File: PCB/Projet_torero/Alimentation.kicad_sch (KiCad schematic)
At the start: 17 parts, among them IC501 MP1475SGJ-P, J2 Conn_01x02, SW3 SW_DPDT_x2, U2 BU33SD5WG-TR

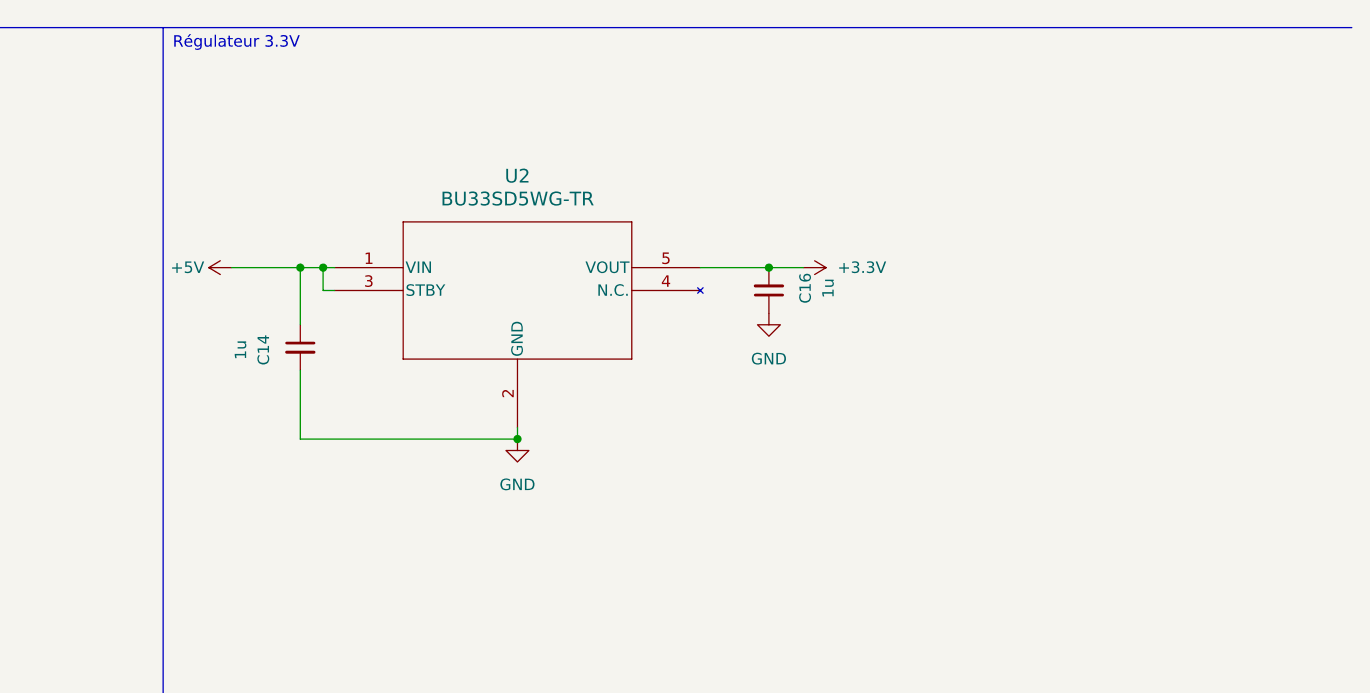
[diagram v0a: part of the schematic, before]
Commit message: review sch
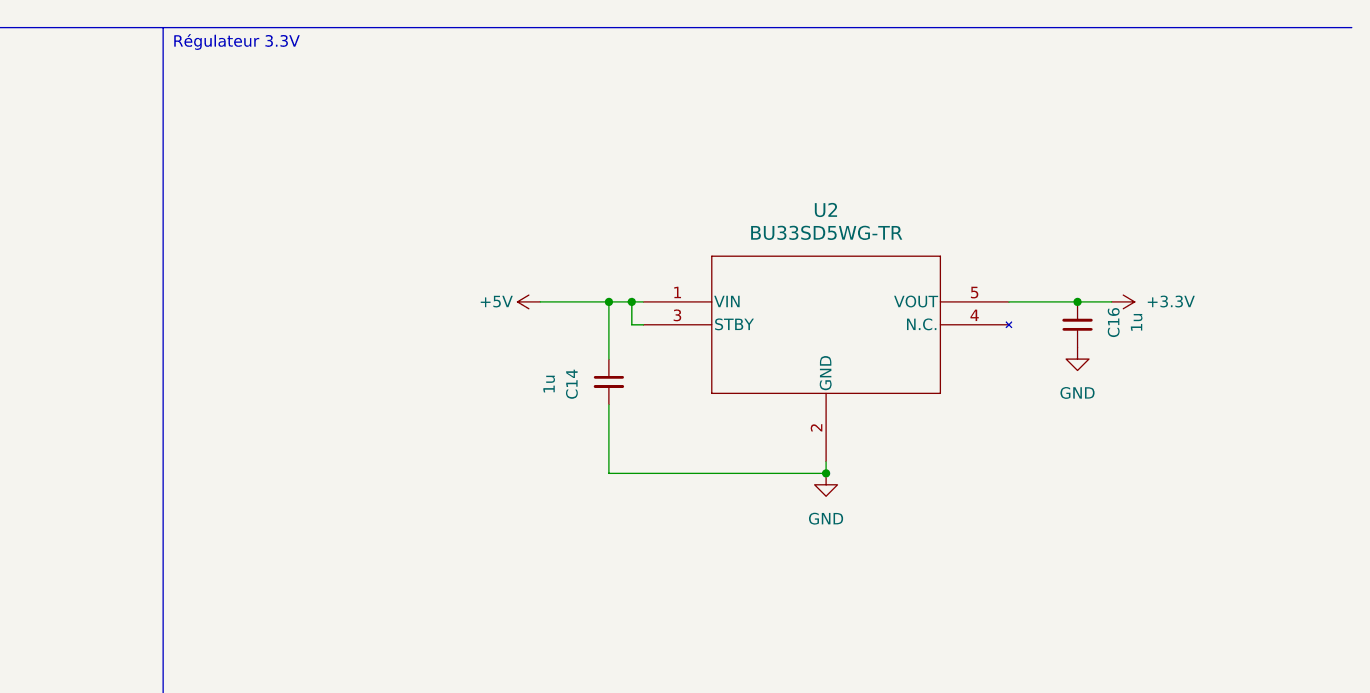
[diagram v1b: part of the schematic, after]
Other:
- moved on the sheet: C14, C16, U2
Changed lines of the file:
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@@
 	(paper "A4")
 	(junction
-		(at 171.45 116.84)
+		(at 205.74 120.65)
 		(diameter 0)
 		(color 0 0 0 0)
@@
 	)
 	(junction
-		(at 168.91 116.84)
+		(at 203.2 120.65)
 		(diameter 0)
 		(color 0 0 0 0)
 	)
 	(junction
-		(at 220.98 116.84)
+		(at 255.27 120.65)
 		(diameter 0)
 		(color 0 0 0 0)
@@
 	)
 	(junction
-		(at 193.04 135.89)
+		(at 227.33 139.7)
 		(diameter 0)
 		(color 0 0 0 0)
@@
 	(wire
 		(pts
-			(xy 168.91 116.84) (xy 168.91 123.19)
+			(xy 203.2 120.65) (xy 203.2 127)
 		)
 		(stroke
@@
 	(wire
 		(pts
-			(xy 168.91 135.89) (xy 193.04 135.89)
+			(xy 203.2 139.7) (xy 227.33 139.7)
 		)
 		(stroke
@@
 	(wire
 		(pts
-			(xy 168.91 128.27) (xy 168.91 135.89)
+			(xy 203.2 132.08) (xy 203.2 139.7)
 		)
 		(stroke
@@
 	(wire
 		(pts
-			(xy 220.98 116.84) (xy 224.79 116.84)
+			(xy 255.27 120.65) (xy 259.08 120.65)
 		)
 		(stroke
@@
 	(wire
 		(pts
-			(xy 213.36 116.84) (xy 220.98 116.84)
+			(xy 247.65 120.65) (xy 255.27 120.65)
 		)
 		(stroke
@@
 	(wire
 		(pts
-			(xy 168.91 116.84) (xy 171.45 116.84)
+			(xy 203.2 120.65) (xy 205.74 120.65)
 		)
 		(stroke
@@
 	(wire
 		(pts
-			(xy 193.04 134.62) (xy 193.04 135.89)
+			(xy 227.33 138.43) (xy 227.33 139.7)
 		)
 		(stroke
@@
 	(wire
 		(pts
-			(xy 171.45 116.84) (xy 171.45 119.38)
+			(xy 205.74 120.65) (xy 205.74 123.19)
 		)
 		(stroke
@@
 	(wire
 		(pts
-			(xy 161.29 116.84) (xy 168.91 116.84)
+			(xy 195.58 120.65) (xy 203.2 120.65)
 		)
 		(stroke
@@
 	(wire
 		(pts
-			(xy 171.45 119.38) (xy 172.72 119.38)
+			(xy 205.74 123.19) (xy 207.01 123.19)
 		)
 		(stroke
@@
 	(wire
 		(pts
-			(xy 171.45 116.84) (xy 172.72 116.84)
+			(xy 205.74 120.65) (xy 207.01 120.65)
 		)
 		(stroke
@@
 	(symbol
 		(lib_id "power:+3.3V")
-		(at 224.79 116.84 270)
+		(at 259.08 120.65 270)
 		(unit 1)
 		(exclude_from_sim no)
@@
 		(fields_autoplaced yes)
 		(property "Reference" "#PWR028"
-			(at 220.98 116.84 0)
+			(at 255.27 120.65 0)
 			(effects
 				(font
@@
 		)
 		(property "Value" "+3.3V"
-			(at 228.6 116.8399 90)
+			(at 262.89 120.6499 90)
 			(effects
 				(font
@@
 		)
 		(property "Footprint" ""
-			(at 224.79 116.84 0)
+			(at 259.08 120.65 0)
 			(effects
 				(font
@@
 		)
 		(property "Datasheet" ""
-			(at 224.79 116.84 0)
+			(at 259.08 120.65 0)
 			(effects
 				(font
@@
 		)
 		(property "Description" "Power symbol creates a global label with name \"+3.3V\""
-			(at 224.79 116.84 0)
+			(at 259.08 120.65 0)
 			(effects
 				(font
@@
 	(symbol
 		(lib_id "power:GND")
-		(at 220.98 121.92 0)
+		(at 255.27 125.73 0)
 		(unit 1)
 		(exclude_from_sim no)
@@
 		(fields_autoplaced yes)
 		(property "Reference" "#PWR025"
-			(at 220.98 128.27 0)
+			(at 255.27 132.08 0)
 			(effects
 				(font
@@
 		)
 		(property "Value" "GND"
-			(at 220.98 127 0)
+			(at 255.27 130.81 0)
 			(effects
 				(font
@@
 		)
 		(property "Footprint" ""
-			(at 220.98 121.92 0)
+			(at 255.27 125.73 0)
 			(effects
 				(font
@@
 		)
 		(property "Datasheet" ""
-			(at 220.98 121.92 0)
+			(at 255.27 125.73 0)
 			(effects
 				(font
@@
 		)
 		(property "Description" "Power symbol creates a global label with name \"GND\" , ground"
-			(at 220.98 121.92 0)
+			(at 255.27 125.73 0)
 			(effects
 				(font
@@
 	(symbol
 		(lib_id "2024-10-01_06-18-21:BU33SD5WG-TR")
-		(at 172.72 116.84 0)
+		(at 207.01 120.65 0)
 		(unit 1)
 		(exclude_from_sim no)
@@
 		(fields_autoplaced yes)
 		(property "Reference" "U2"
-			(at 193.04 106.68 0)
+			(at 227.33 110.49 0)
 			(effects
 				(font
@@
 		)
 		(property "Value" "BU33SD5WG-TR"
-			(at 193.04 109.22 0)
+			(at 227.33 113.03 0)
 			(effects
 				(font
@@
 		)
 		(property "Footprint" "SSOP5_ROM"
-			(at 172.72 116.84 0)
+			(at 207.01 120.65 0)
 			(effects
 				(font
@@
 		)
 		(property "Datasheet" "BU33SD5WG-TR"
-			(at 172.72 116.84 0)
+			(at 207.01 120.65 0)
 			(effects
 				(font
@@
 		)
 		(property "Description" ""
-			(at 172.72 116.84 0)
+			(at 207.01 120.65 0)
 			(effects
 				(font
@@
 	(symbol
 		(lib_id "Device:C_Small")
-		(at 168.91 125.73 0)
+		(at 203.2 129.54 0)
 		(unit 1)
 		(exclude_from_sim no)
@@
 		(dnp no)
 		(property "Reference" "C14"
-			(at 164.846 125.984 90)
+			(at 199.136 129.794 90)
 			(effects
 				(font
@@
 		)
 		(property "Value" "1u"
-			(at 162.306 125.984 90)
+			(at 196.596 129.794 90)
 			(effects
 				(font
@@
 		)
 		(property "Footprint" ""
-			(at 168.91 125.73 0)
+			(at 203.2 129.54 0)
 			(effects
 				(font
@@
 		)
 		(property "Datasheet" "~"
-			(at 168.91 125.73 0)
+			(at 203.2 129.54 0)
 			(effects
 				(font
@@
 		)
 		(property "Description" "Unpolarized capacitor, small symbol"
-			(at 168.91 125.73 0)
+			(at 203.2 129.54 0)
 			(effects
 				(font
@@
 	(symbol
 		(lib_id "Device:C_Small")
-		(at 220.98 119.38 180)
+		(at 255.27 123.19 180)
 		(unit 1)
 		(exclude_from_sim no)
@@
 		(dnp no)
 		(property "Reference" "C16"
-			(at 225.044 119.126 90)
+			(at 259.334 122.936 90)
 			(effects
 				(font
@@
 		)
 		(property "Value" "1u"
-			(at 227.584 119.126 90)
+			(at 261.874 122.936 90)
 			(effects
 				(font
@@
 		)
 		(property "Footprint" ""
-			(at 220.98 119.38 0)
+			(at 255.27 123.19 0)
 			(effects
 				(font
@@
 		)
 		(property "Datasheet" "~"
-			(at 220.98 119.38 0)
+			(at 255.27 123.19 0)
 			(effects
 				(font
@@
 		)
 		(property "Description" "Unpolarized capacitor, small symbol"
-			(at 220.98 119.38 0)
+			(at 255.27 123.19 0)
 			(effects
 				(font
@@
 	(symbol
 		(lib_id "power:GND")
-		(at 193.04 135.89 0)
+		(at 227.33 139.7 0)
 		(unit 1)
 		(exclude_from_sim no)
@@
 		(fields_autoplaced yes)
 		(property "Reference" "#PWR022"
-			(at 193.04 142.24 0)
+			(at 227.33 146.05 0)
 			(effects
 				(font
@@
 		)
 		(property "Value" "GND"
-			(at 193.04 140.97 0)
+			(at 227.33 144.78 0)
 			(effects
 				(font
@@
 		)
 		(property "Footprint" ""
-			(at 193.04 135.89 0)
+			(at 227.33 139.7 0)
 			(effects
 				(font
@@
 		)
 		(property "Datasheet" ""
-			(at 193.04 135.89 0)
+			(at 227.33 139.7 0)
 			(effects
 				(font
@@
 		)
 		(property "Description" "Power symbol creates a global label with name \"GND\" , ground"
-			(at 193.04 135.89 0)
+			(at 227.33 139.7 0)
 			(effects
 				(font
@@
 	(symbol
 		(lib_id "power:+5V")
-		(at 161.29 116.84 90)
+		(at 195.58 120.65 90)
 		(unit 1)
 		(exclude_from_sim no)
@@
 		(dnp no)
 		(property "Reference" "#PWR026"
-			(at 165.1 116.84 0)
+			(at 199.39 120.65 0)
 			(effects
 				(font
@@
 		)
 		(property "Value" "+5V"
-			(at 158.242 116.84 90)
+			(at 192.532 120.65 90)
 			(effects
 				(font
@@
 		)
 		(property "Footprint" ""
-			(at 161.29 116.84 0)
+			(at 195.58 120.65 0)
 			(effects
 				(font
@@
 		)
 		(property "Datasheet" ""
-			(at 161.29 116.84 0)
+			(at 195.58 120.65 0)
 			(effects
 				(font
@@
 		)
 		(property "Description" "Power symbol creates a global label with name \"+5V\""
-			(at 161.29 116.84 0)
-			(effects
-				(font
+			(at 195.58 120.65 0)
+			(effects
+				(font
